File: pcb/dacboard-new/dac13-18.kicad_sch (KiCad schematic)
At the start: 30 parts, among them U34 AD8676xR, U35 AD8676xR, U36 AD8676xR, U37 AD8676xR, U38 AD5791BRUZ, U39 AD5791BRUZ, U40 AD5791BRUZ, U41 AD5791BRUZ, U42 AD8676xR, U43 AD8676xR, U44 AD5791BRUZ, U45 AD5791BRUZ

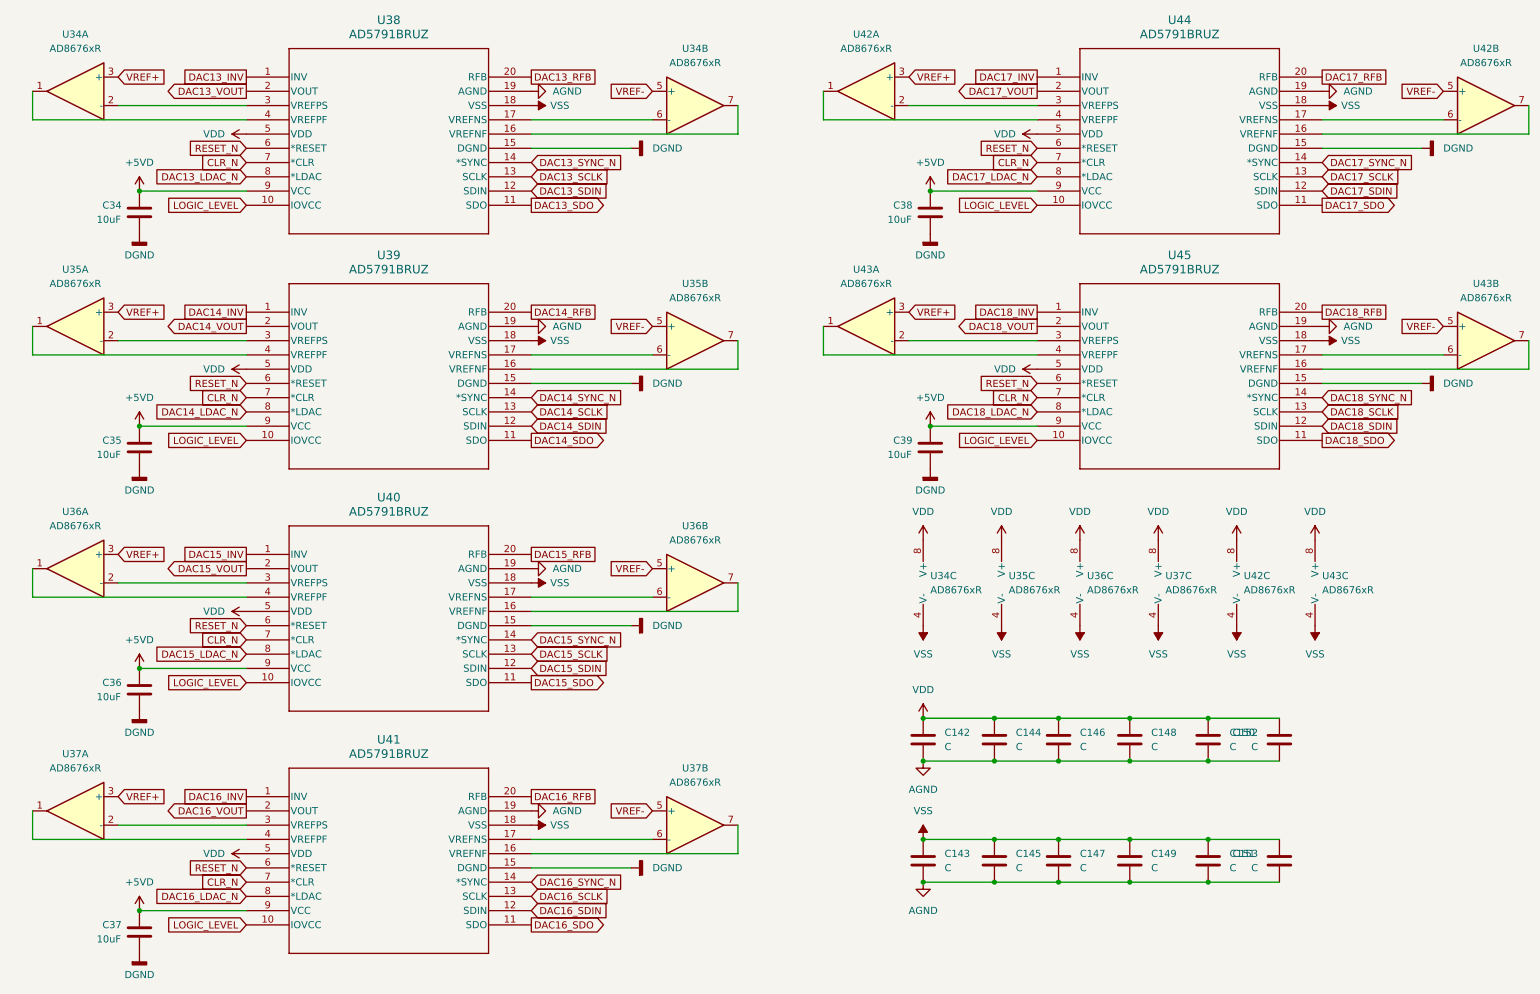
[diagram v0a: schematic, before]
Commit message: new pcb progress
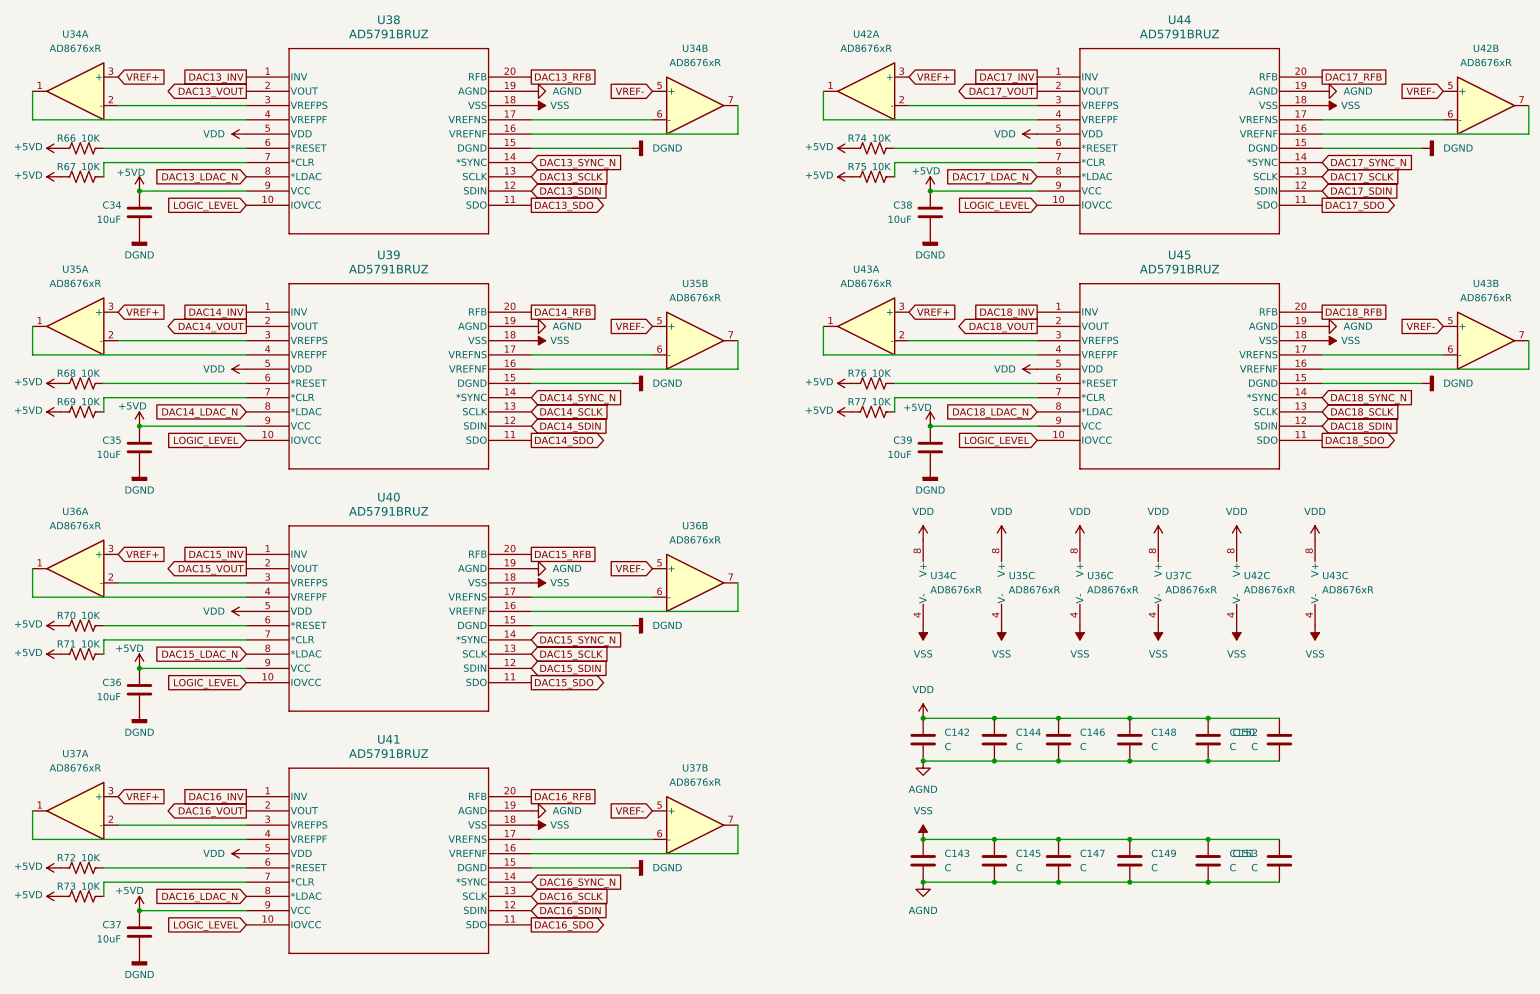
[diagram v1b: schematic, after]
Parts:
- added R66, R67, R68, R69, R70, R71, R72, R73, R74, R75, R76, R77: 10K, Resistor_SMD:R_0402_1005Metric_Pad0.72x0.64mm_HandSolder, symbol Device:R_US
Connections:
- net +5VD: now also R66.1, R67.1, R68.1, R69.1, R70.1, R71.1, R72.1, R73.1, R74.1, R75.1, R76.1, R77.1
- removed net CLR_N: U38.7 (*CLR), U39.7 (*CLR), U40.7 (*CLR), U41.7 (*CLR), U44.7 (*CLR), U45.7 (*CLR)
- removed net RESET_N: U38.6 (*RESET), U39.6 (*RESET), U40.6 (*RESET), U41.6 (*RESET), U44.6 (*RESET), U45.6 (*RESET)
- new net: R69.2, U39.7 (*CLR)
- new net: R76.2, U45.6 (*RESET)
- new net: R72.2, U41.6 (*RESET)
- new net: R70.2, U40.6 (*RESET)
- new net: R71.2, U40.7 (*CLR)
- new net: R66.2, U38.6 (*RESET)
- new net: R67.2, U38.7 (*CLR)
- new net: R75.2, U44.7 (*CLR)
- new net: R74.2, U44.6 (*RESET)
- new net: R77.2, U45.7 (*CLR)
- new net: R73.2, U41.7 (*CLR)
- new net: R68.2, U39.6 (*RESET)
